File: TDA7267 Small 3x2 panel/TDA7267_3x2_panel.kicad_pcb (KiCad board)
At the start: 2 copper layers, 88 x 97 mm, 108 parts, among them U1 TDA7267

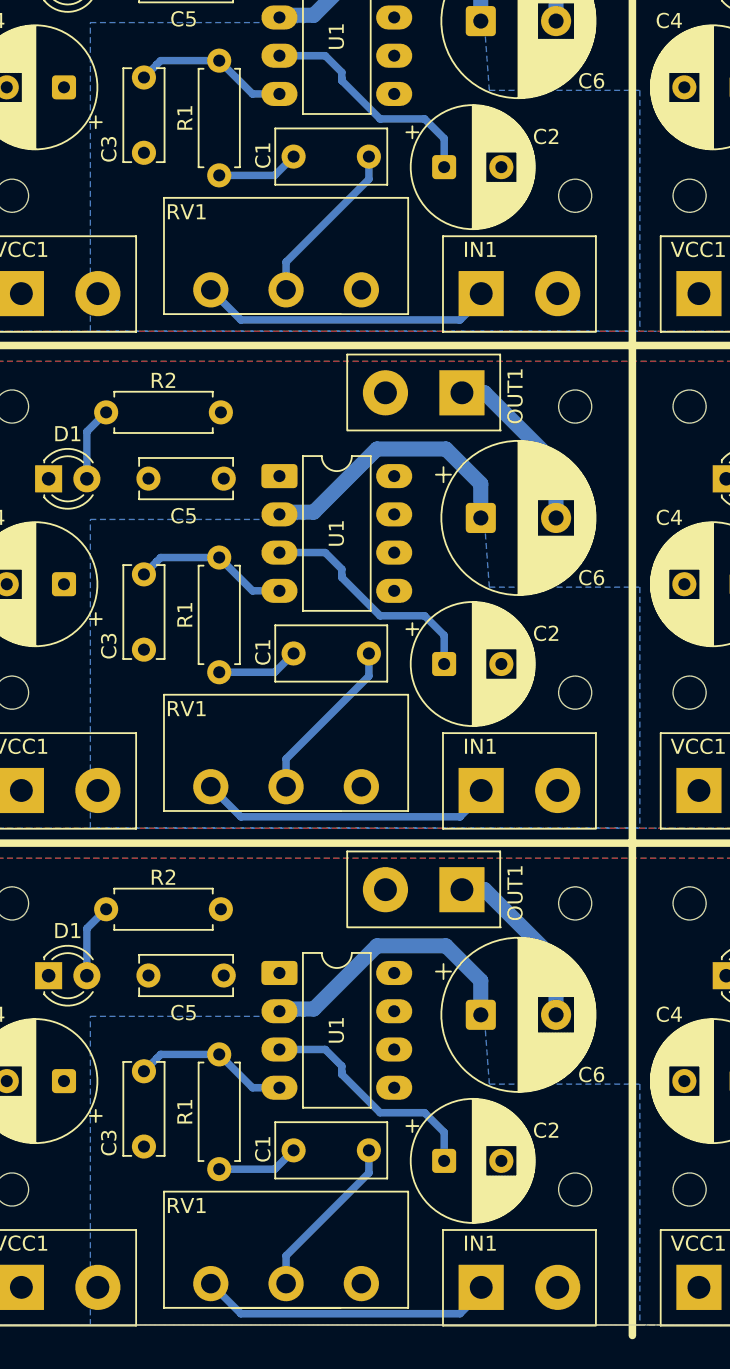
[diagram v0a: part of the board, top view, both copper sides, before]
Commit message: Tweaks
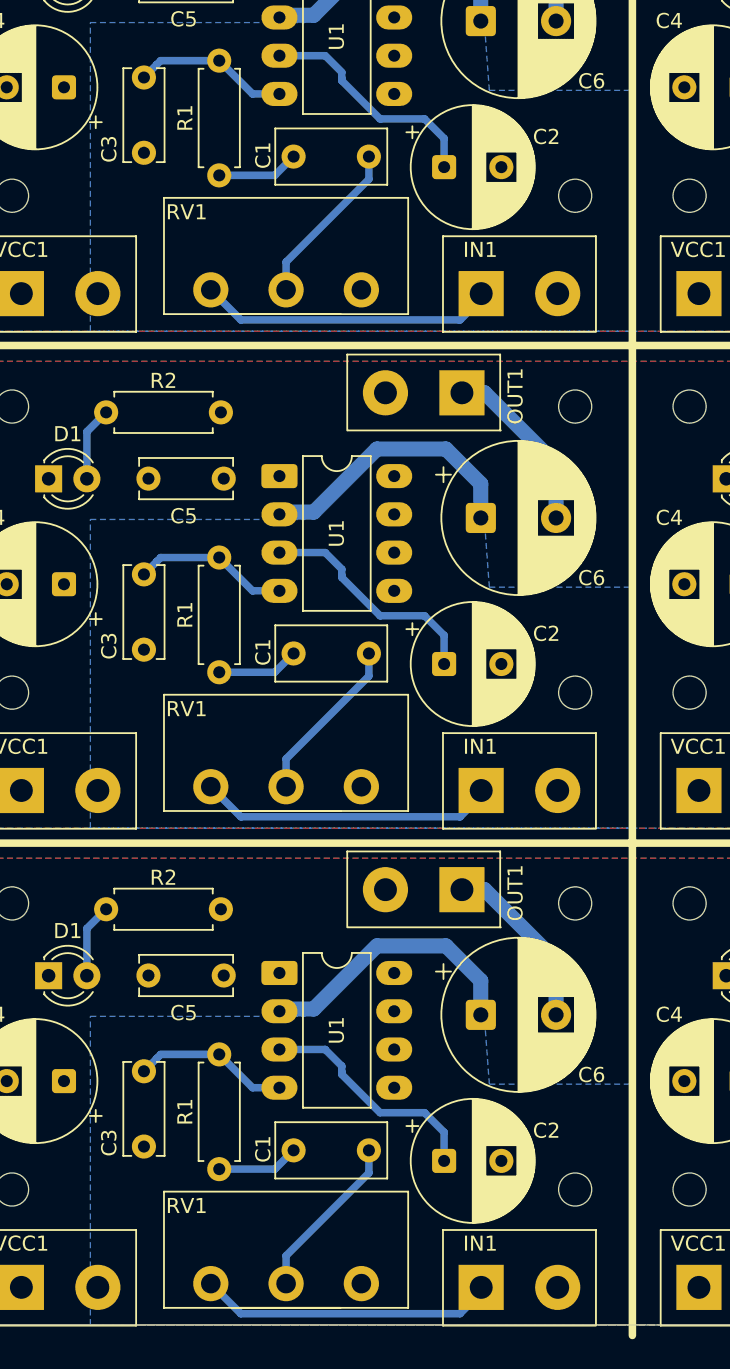
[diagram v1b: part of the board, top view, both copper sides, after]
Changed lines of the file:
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@@
 				(thickness 0.035)
 			)
-			(layer "dielectric 1"
+			(layer "dielectric 2"
 				(type "core")
 				(thickness 1.51)
@@
 		(hatch edge 0.5)
 		(connect_pads yes
-			(clearance 0.5)
+			(clearance 0.3)
 		)
 		(min_thickness 0.25)
@@
 		(hatch edge 0.5)
 		(connect_pads yes
-			(clearance 0.5)
+			(clearance 0.3)
 		)
 		(min_thickness 0.25)
@@
 		(hatch edge 0.5)
 		(connect_pads yes
-			(clearance 0.5)
+			(clearance 0.3)
 		)
 		(min_thickness 0.25)
@@
 		(priority 1)
 		(connect_pads yes
-			(clearance 0.5)
+			(clearance 0.3)
 		)
 		(min_thickness 0.25)
@@
 		(priority 1)
 		(connect_pads yes
-			(clearance 0.5)
+			(clearance 0.3)
 		)
 		(min_thickness 0.25)
@@
 			(pts
 				(xy 90.75 72.65) (xy 90.75 52.15) (xy 105 52.15) (xy 110 47.4) (xy 114.5 47.4) (xy 116.75 49.9)
-				(xy 117.25 56.65) (xy 127.25 56.65) (xy 127.25 72.65)
+				(xy 117.25 56.65) (xy 126.75 56.65) (xy 126.75 72.65)
 			)
 		)
@@
 		(hatch edge 0.5)
 		(connect_pads yes
-			(clearance 0.5)
+			(clearance 0.3)
 		)
 		(min_thickness 0.25)
@@
 		(hatch edge 0.5)
 		(connect_pads yes
-			(clearance 0.5)
+			(clearance 0.3)
 		)
 		(min_thickness 0.25)
@@
 		(priority 1)
 		(connect_pads yes
-			(clearance 0.5)
+			(clearance 0.3)
 		)
 		(min_thickness 0.25)
@@
 			(pts
 				(xy 90.75 105.65) (xy 90.75 85.15) (xy 105 85.15) (xy 110 80.4) (xy 114.5 80.4) (xy 116.75 82.9)
-				(xy 117.25 89.65) (xy 127.25 89.65) (xy 127.25 105.65)
+				(xy 117.25 89.65) (xy 126.75 89.65) (xy 126.75 105.65)
 			)
 		)
@@
 		(priority 1)
 		(connect_pads yes
-			(clearance 0.5)
+			(clearance 0.3)
 		)
 		(min_thickness 0.25)
@@
 			(pts
 				(xy 90.75 138.65) (xy 90.75 118.15) (xy 105 118.15) (xy 110 113.4) (xy 114.5 113.4) (xy 116.75 115.9)
-				(xy 117.25 122.65) (xy 127.25 122.65) (xy 127.25 138.65)
+				(xy 117.25 122.65) (xy 126.75 122.65) (xy 126.75 138.65)
 			)
 		)
@@
 		(priority 1)
 		(connect_pads yes
-			(clearance 0.5)
+			(clearance 0.3)
 		)
 		(min_thickness 0.25)
@@
 		(hatch edge 0.5)
 		(connect_pads yes
-			(clearance 0.5)
+			(clearance 0.3)
 		)
 		(min_thickness 0.25)
@@
 		(priority 1)
 		(connect_pads yes
-			(clearance 0.5)
+			(clearance 0.3)
 		)
 		(min_thickness 0.25)
